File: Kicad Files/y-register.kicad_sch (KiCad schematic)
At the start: 20 parts, among them U1 74LS245, U2 74LS173, U3 74LS173

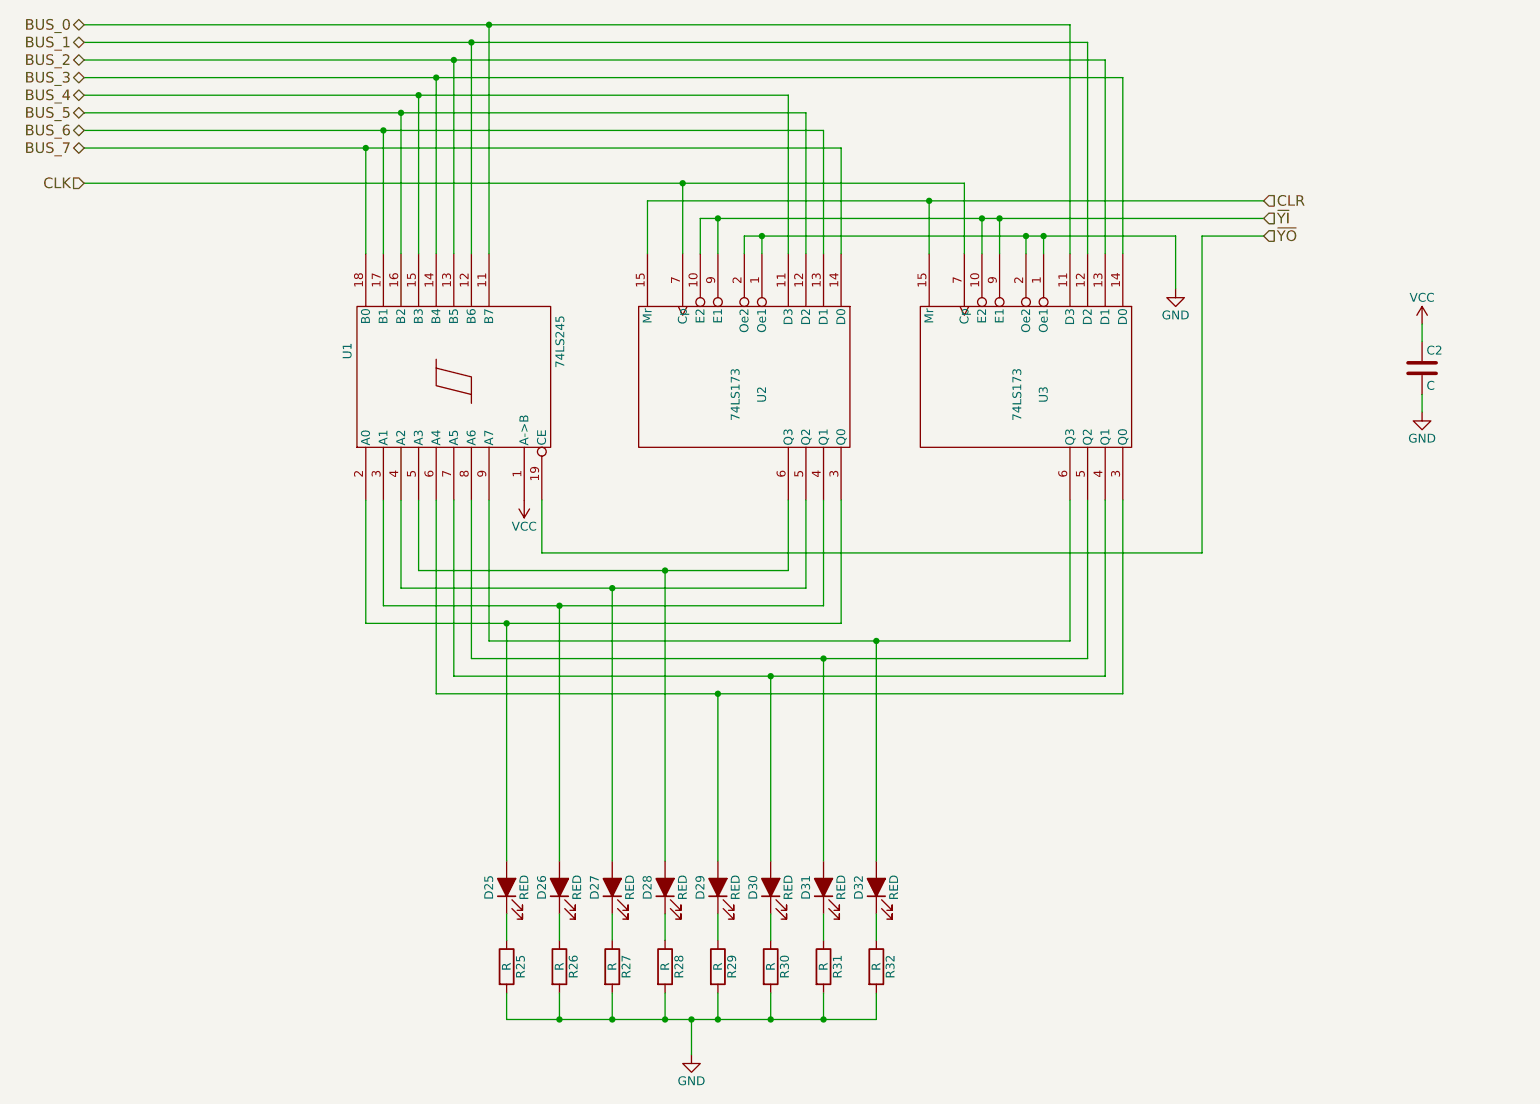
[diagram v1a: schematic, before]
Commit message: updated library
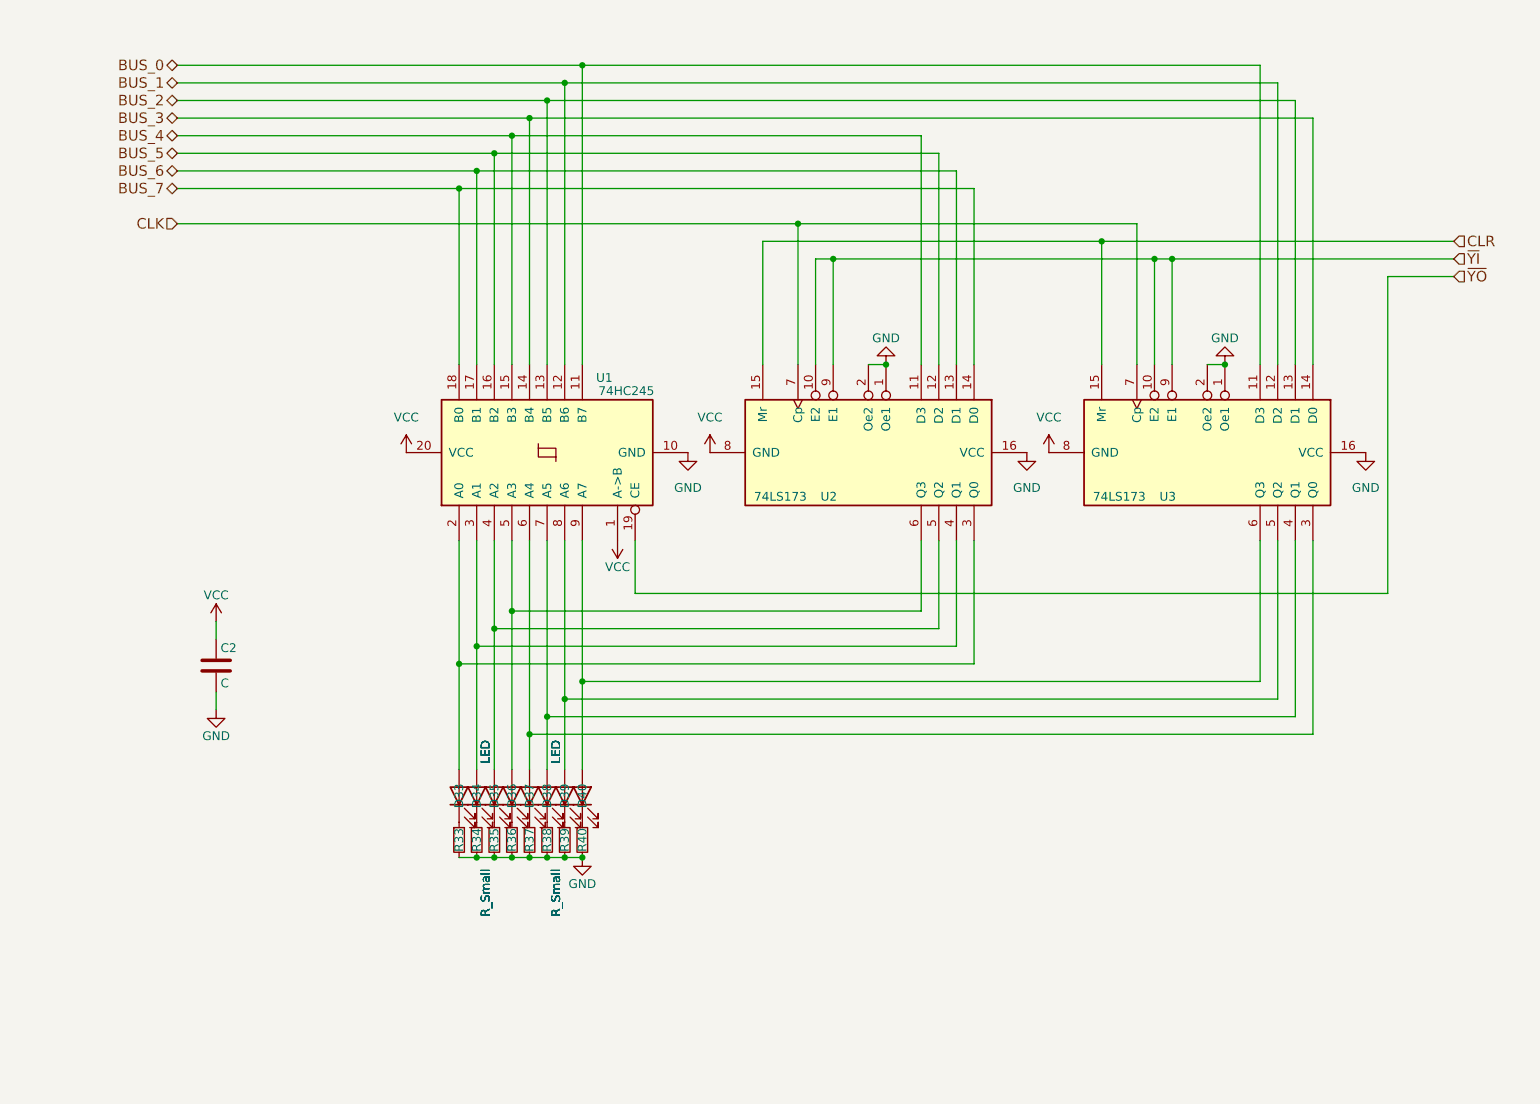
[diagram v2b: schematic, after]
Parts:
- removed D25, D26, D27, D28, D29, D30, D31, D32: RED, LED_THT:LED_D5.0mm, symbol 8bit-computer-rescue:LED_ALT-Device
- removed R25, R26, R27, R28, R29, R30, R31, R32: R, Resistor_THT:R_Axial_DIN0207_L6.3mm_D2.5mm_P7.62mm_Horizontal, symbol Device:R
- removed U1: 74LS245, Package_DIP:DIP-20_W7.62mm, symbol 8bit-computer-rescue:74LS245-8bit-computer-rescue
- removed U2, U3: 74LS173, Package_DIP:DIP-16_W7.62mm, symbol 8bit-computer-rescue:74LS173-8bit-computer-rescue
- added D33, D34, D35, D36, D37, D38, D39, D40: LED, symbol Device:LED
- added R33, R34, R35, R36, R37, R38, R39, R40: R_Small, symbol Device:R_Small
- added U1: 74HC245, symbol 74xx:74HC245
- added U2, U3: 74LS173, symbol 74xx:74LS173
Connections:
- net BUS_0: now also U1.11 (B7), U3.11 (D3)
- net BUS_1: now also U1.12 (B6), U3.12 (D2)
- net BUS_2: now also U1.13 (B5), U3.13 (D1)
- net BUS_3: now also U1.14 (B4), U3.14 (D0)
- net BUS_4: now also U1.15 (B3), U2.11 (D3)
- net BUS_5: now also U1.16 (B2), U2.12 (D2)
- net BUS_6: now also U1.17 (B1), U2.13 (D1)
- net BUS_7: now also U1.18 (B0), U2.14 (D0)
- net CLK: now also U2.7 (Cp), U3.7 (Cp)
- net CLR: now also U2.15 (Mr), U3.15 (Mr)
- net GND: now also R33.2, R34.2, R35.2, R36.2, R37.2, R38.2, R39.2, R40.2, U1.10 (GND), U2.1 (Oe1), U2.16 (VCC), U2.2 (Oe2), U3.1 (Oe1), U3.16 (VCC), U3.2 (Oe2)
- net VCC: now also U1.1 (A->B), U1.20 (VCC), U2.8 (GND), U3.8 (GND)
- net ~{YI}: now also U2.10 (E2), U2.9 (E1), U3.10 (E2), U3.9 (E1)
- net ~{YO}: now also U1.19 (CE)
- new net: D33.2 (A), U1.2 (A0), U2.3 (Q0)
- new net: D34.2 (A), U1.3 (A1), U2.4 (Q1)
- new net: D35.2 (A), U1.4 (A2), U2.5 (Q2)
- new net: D36.2 (A), U1.5 (A3), U2.6 (Q3)
- new net: D33.1 (K), R33.1
- new net: D35.1 (K), R35.1
- new net: D38.1 (K), R38.1
- new net: D38.2 (A), U1.7 (A5), U3.4 (Q1)
- new net: D37.1 (K), R37.1
- new net: D34.1 (K), R34.1
- new net: D36.1 (K), R36.1
- new net: D40.1 (K), R40.1
- new net: D37.2 (A), U1.6 (A4), U3.3 (Q0)
- new net: D40.2 (A), U1.9 (A7), U3.6 (Q3)
- new net: D39.2 (A), U1.8 (A6), U3.5 (Q2)
- new net: D39.1 (K), R39.1
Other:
- moved on the sheet: C2

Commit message: im sooo stupiiid
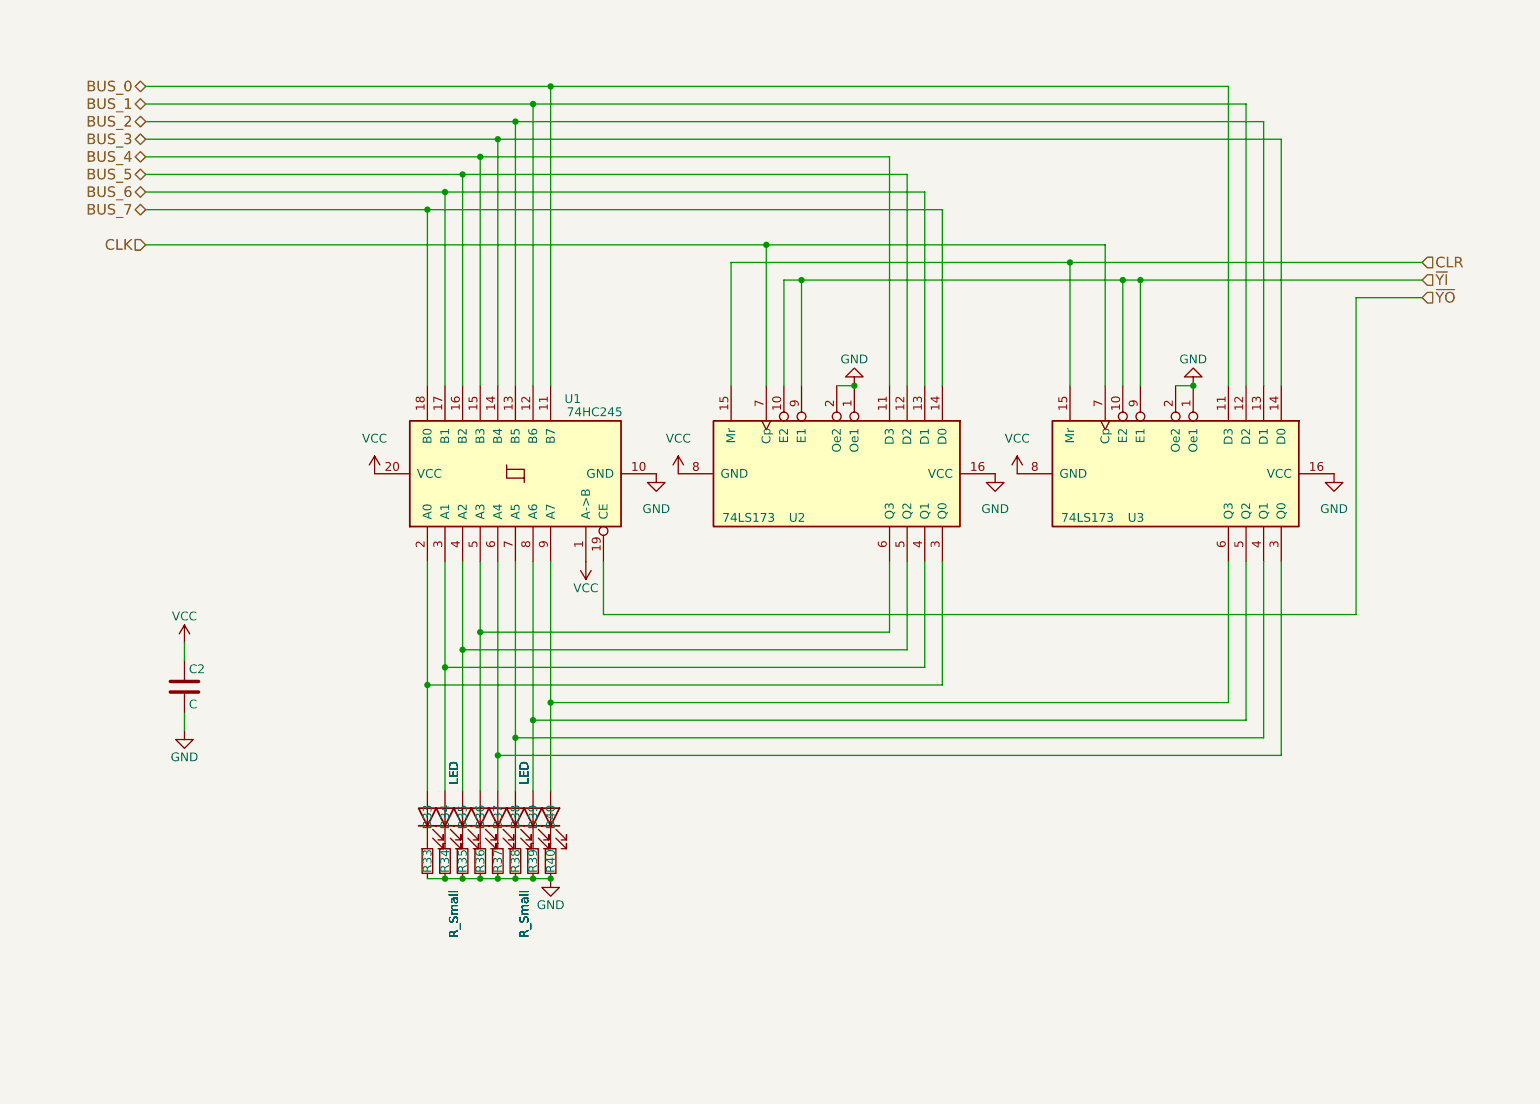
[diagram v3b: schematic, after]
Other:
- moved on the sheet: C2, D33, D34, D35, D36, D37, D38, D39, D40, R33, R34, R35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
